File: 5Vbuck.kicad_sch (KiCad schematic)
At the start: 16 parts, among them U3 LM5146RGYR

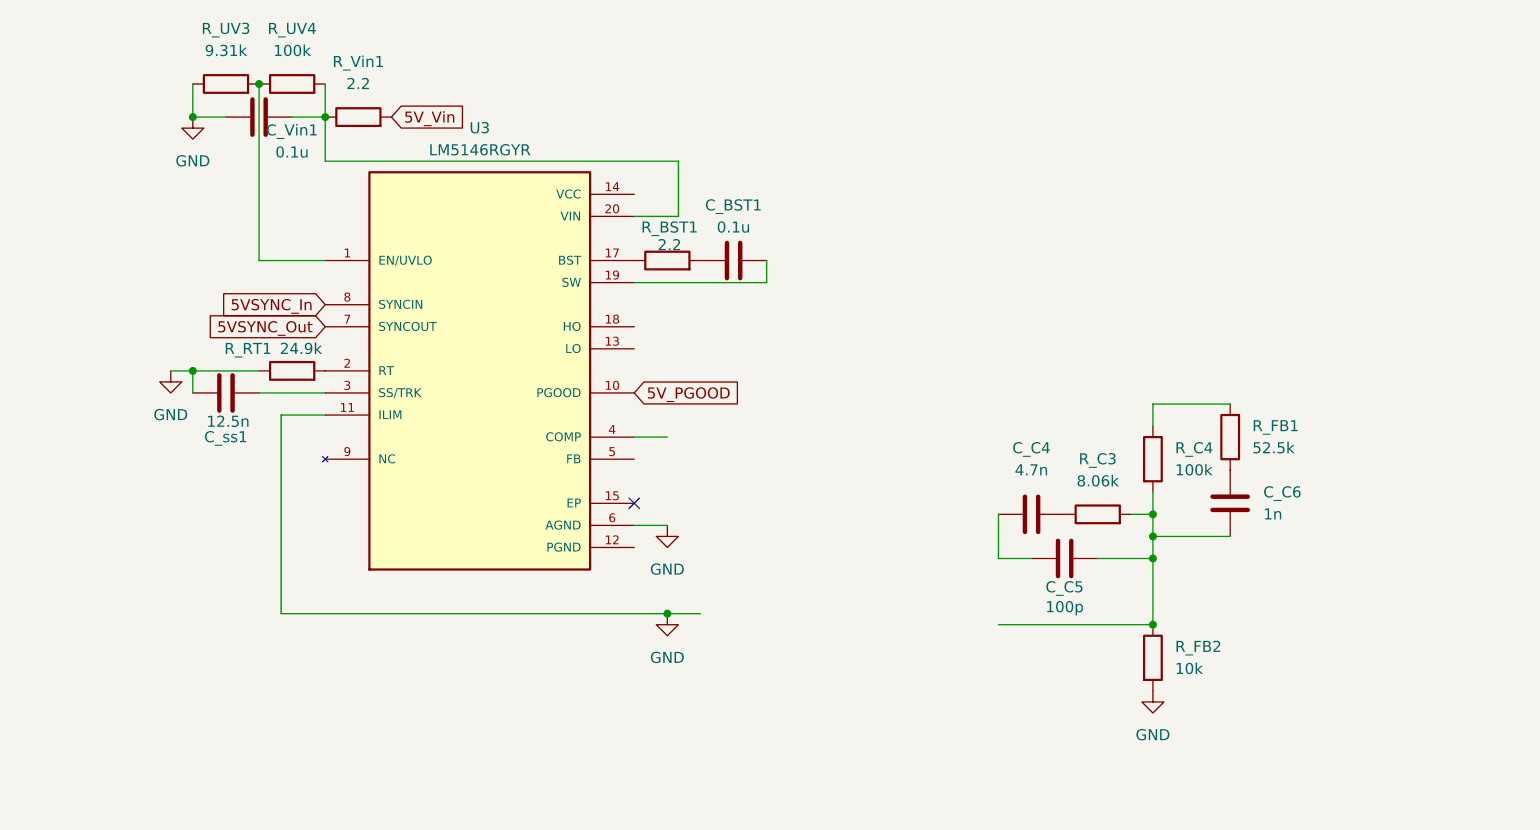
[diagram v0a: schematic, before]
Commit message: navn på alle komp i 5V
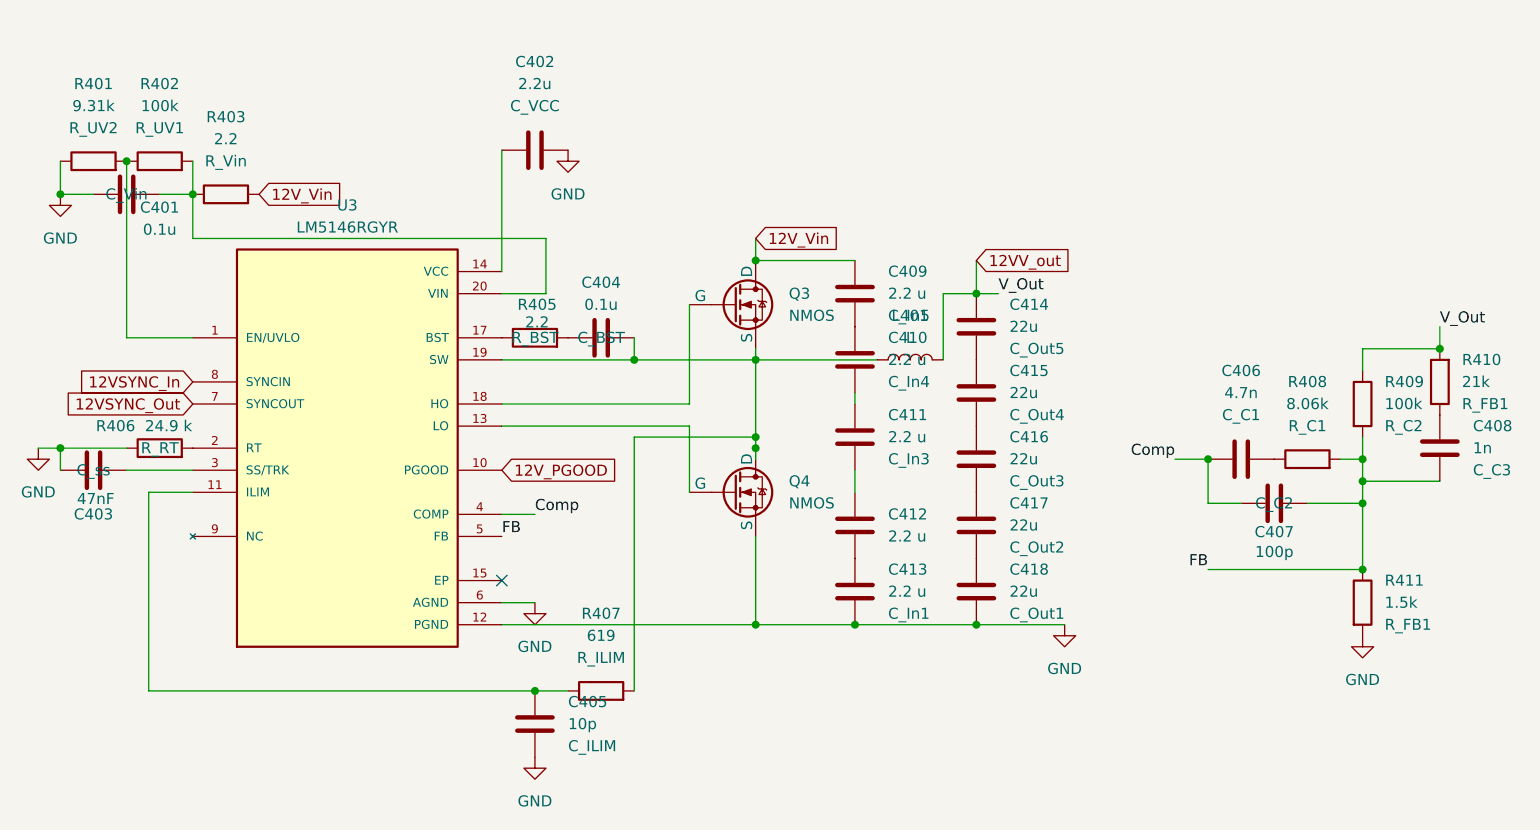
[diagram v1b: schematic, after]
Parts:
- removed C_BST1, C_Vin1: 0.1u, symbol Device:C
- removed C_C4: 4.7n, symbol Device:C
- removed C_C5: 100p, symbol Device:C
- removed C_C6: 1n, symbol Device:C
- removed C_ss1: 12.5n, symbol Device:C
- removed R_BST1, R_Vin1: 2.2, symbol Device:R
- removed R_C3: 8.06k, symbol Device:R
- removed R_C4, R_UV4: 100k, symbol Device:R
- removed R_FB1: 52.5k, symbol Device:R
- removed R_FB2: 10k, symbol Device:R
- removed R_RT1: 24.9k, symbol Device:R
- removed R_UV3: 9.31k, symbol Device:R
- added C401, C404: 0.1u, symbol Device:C
- added C402: 2.2u, symbol Device:C
- added C403: 47nF, symbol Device:C
- added C405: 10p, symbol Device:C
- added C406: 4.7n, symbol Device:C
- added C407: 100p, symbol Device:C
- added C408: 1n, symbol Device:C
- added C409, C410, C411, C412, C413: 2.2 u, symbol Device:C
- added C414, C415, C416, C417, C418: 22u, symbol Device:C
- added L401: L, Package_SO:SSOP-16_3.9x4.9mm_P0.635mm, symbol Device:L
- added Q3, Q4: NMOS, Package_DFN_QFN:Nordic_AQFN-94-1EP_7x7mm_P0.4mm, symbol Simulation_SPICE:NMOS
- added R401: 9.31k, symbol Device:R
- added R402, R409: 100k, symbol Device:R
- added R403, R405: 2.2, symbol Device:R
- added R406: 24.9 k, symbol Device:R
- added R407: 619, symbol Device:R
- added R408: 8.06k, symbol Device:R
- added R410: 21k, symbol Device:R
- added R411: 1.5k, symbol Device:R
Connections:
- net GND: now also U3.12 (PGND), C401.1, C402.2, C403.1, C405.2, C413.2, C418.2, Q4.3 (S), R401.1, R406.1, R411.2; no longer U3.11 (ILIM)
- net at U3.20 (VIN): now also C401.2, R402.2, R403.1
- net at U3.17 (BST): now also R405.1
- net at U3.19 (SW): now also C404.2, L401.1, Q3.3 (S), Q4.1 (D), R407.2
- net at U3.1 (EN/UVLO): now also R401.2, R402.1
- net at U3.3 (SS/TRK): now also C403.2
- net at U3.13 (LO): now also Q4.2 (G)
- net at U3.14 (VCC): now also C402.1
- net at U3.18 (HO): now also Q3.2 (G)
- net at U3.2 (RT): now also R406.2
- net Comp: now reaches U3.4 (COMP)
- net Comp: now also C406.2, C407.1
- net FB: now reaches U3.5 (FB)
- net FB: now also C407.2, C408.1, R408.2, R409.2, R411.1
- net 5VSYNC_In renamed 12VSYNC_In
- net 5VSYNC_Out renamed 12VSYNC_Out
- net 5V_PGOOD renamed 12V_PGOOD
- new net: C411.2, C412.1
- new net: C412.2, C413.1
- new net: C409.2, C410.1
- new net: C416.2, C417.1
- new net: C417.2, C418.1
- new net: C405.1, R407.1, U3.11 (ILIM)
- new net: C414.2, C415.1
- new net: C404.1, R405.2
- new net: C408.2, R410.1
- new net: C406.1, R408.1
- new net: C415.2, C416.1
- new net: C410.2, C411.1
- new net 12VV_out: C414.1, L401.2, R409.1, R410.2
- new net 12V_Vin: C409.1, Q3.1 (D), R403.2
